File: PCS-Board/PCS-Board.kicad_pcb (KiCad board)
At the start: 2 copper layers, 24 parts, among them J1 DB25_Female_MountingHoles, J2 Conn_01x04, U1 MMPQ2222A, U2 MMPQ2222A, U3 MMPQ2222A, U4 uA7805, U5 ADG715, U6 ADG715

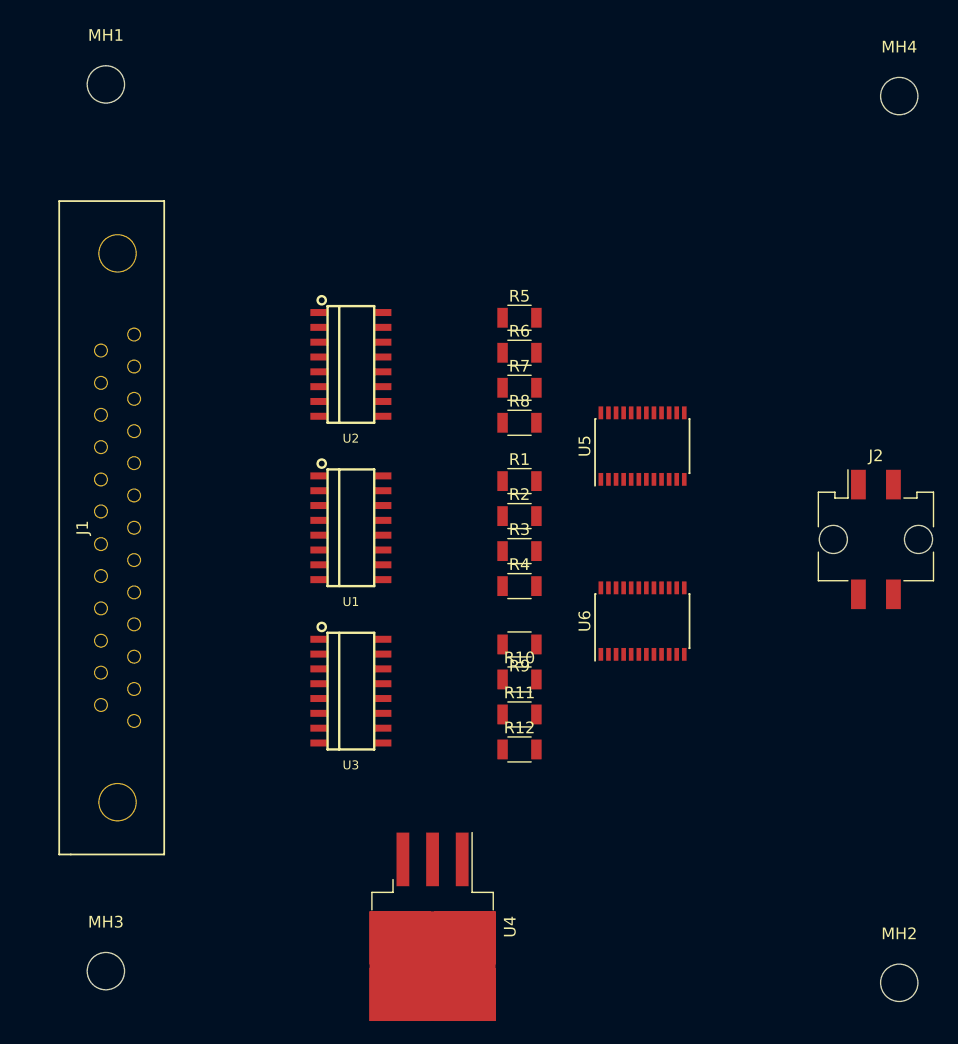
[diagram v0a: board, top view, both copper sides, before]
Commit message: Wiring has begun Im dead inside
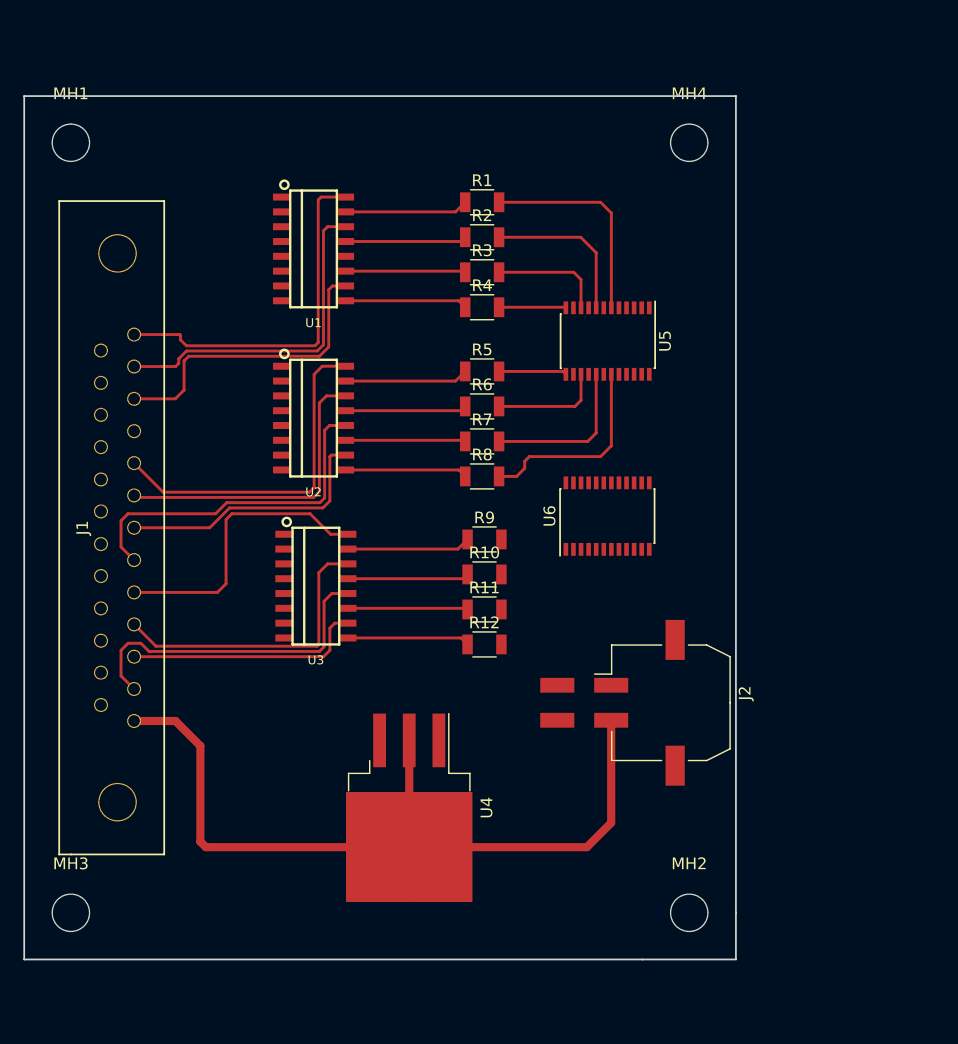
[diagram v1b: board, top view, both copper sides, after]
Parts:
- J2: footprint Connector_Molex:Molex_Micro-Fit_3.0_43045-0415_2x02_P3.00mm_Vertical -> Connectors_Molex:Molex_MicroFit_3.0-43045-0410_04x3.00mm_Angled
- moved J2 28.7 mm to (150.0, 113.0), turned to 270 degrees
- moved U1 24.1 mm to (126.8, 74.1)
- moved R1 24.1 mm to (141.2, 70.1)
- moved R2 24.1 mm to (141.2, 73.1)
- moved R3 24.1 mm to (141.2, 76.1)
- moved R4 24.1 mm to (141.2, 79.1)
- moved MH2 19.0 mm to (159.0, 131.0)
- moved MH4 18.4 mm to (159.0, 65.0)
- moved U4 10.4 mm to (135.0, 122.0)
- moved R10 9.49 mm to (141.4, 102.0)
- moved R11 9.49 mm to (141.4, 105.0)
- moved R12 9.49 mm to (141.4, 108.0)
- moved R9 9.49 mm to (141.4, 99.0), turned to 0 degrees
- moved U3 9.49 mm to (127.0, 103.0)
- moved U5 9.49 mm to (152.0, 82.0), turned to 270 degrees
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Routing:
- net GND: track 0.00 -> 69.0 mm
- net SOLN_PW0: track 0.00 -> 31.2 mm
- net SOLN_PW7: track 0.00 -> 29.8 mm
- net SOLN_PW4: track 0.00 -> 29.3 mm
- net SOLN_PW1: track 0.00 -> 29.0 mm
- net SOLN_PW11: track 0.00 -> 28.1 mm
- net SOLN_PW2: track 0.00 -> 26.4 mm
- net SOLN_PW5: track 0.00 -> 26.2 mm
- net SOLN_PW9: track 0.00 -> 25.6 mm
- net SOLN_PW8: track 0.00 -> 25.0 mm
- net SOLN_PW6: track 0.00 -> 22.9 mm
- net SOLN_PW10: track 0.00 -> 20.6 mm
- net SOLN_EN0: track 0.00 -> 18.1 mm
- net SOLN_EN7: track 0.00 -> 17.2 mm
- net SOLN_EN6: track 0.00 -> 13.7 mm
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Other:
- board outline added: 61 x 74 mm
- net class 12v added: clearance 0.3, trace_width 0.5, via_dia 0.8, via_drill 0.4
- net class GND added: clearance 0.2, trace_width 0.7, via_dia 0.8, via_drill 0.4
